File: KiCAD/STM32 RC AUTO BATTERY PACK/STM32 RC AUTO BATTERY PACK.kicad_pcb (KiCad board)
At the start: 2 copper layers, 147 x 100.2 mm, 9 parts, among them J1 Conn_01x02_Socket, J2 Conn_01x02_Socket, J3 Conn_01x02_Socket

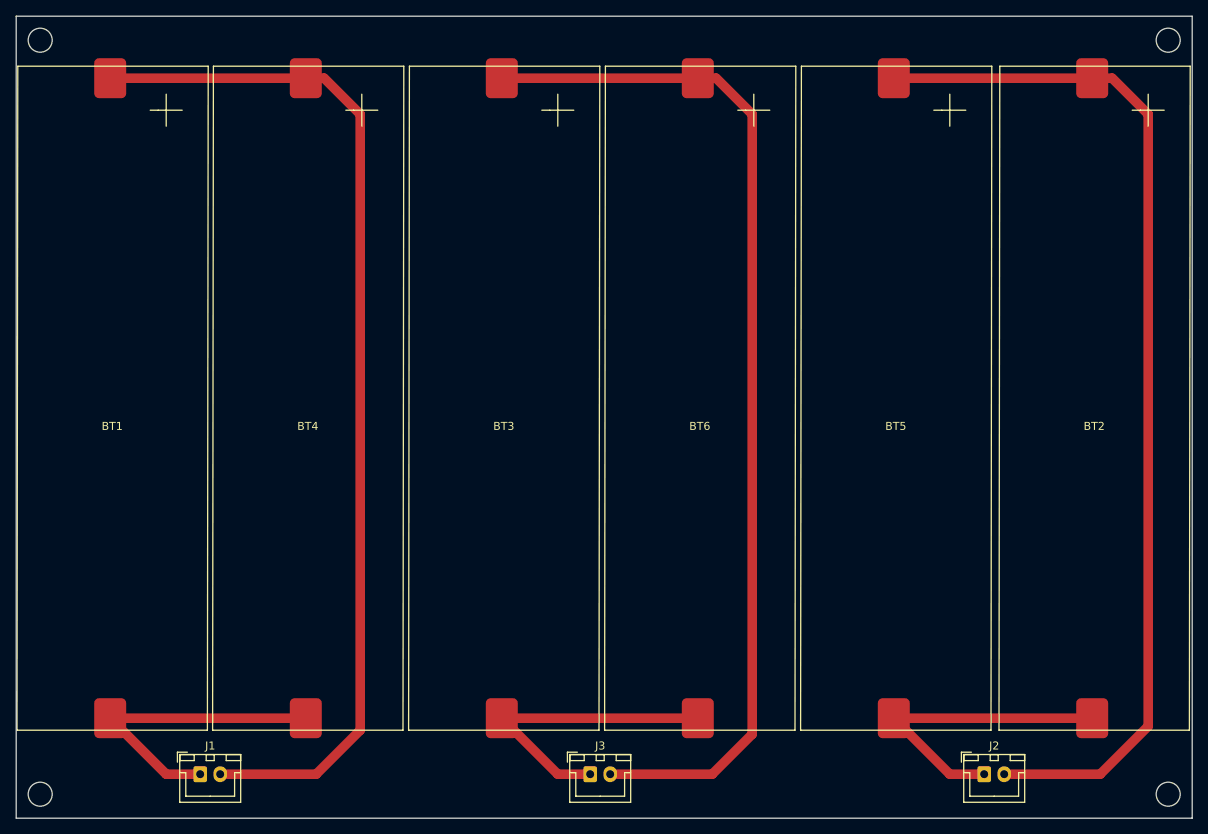
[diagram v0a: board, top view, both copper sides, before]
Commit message: ,
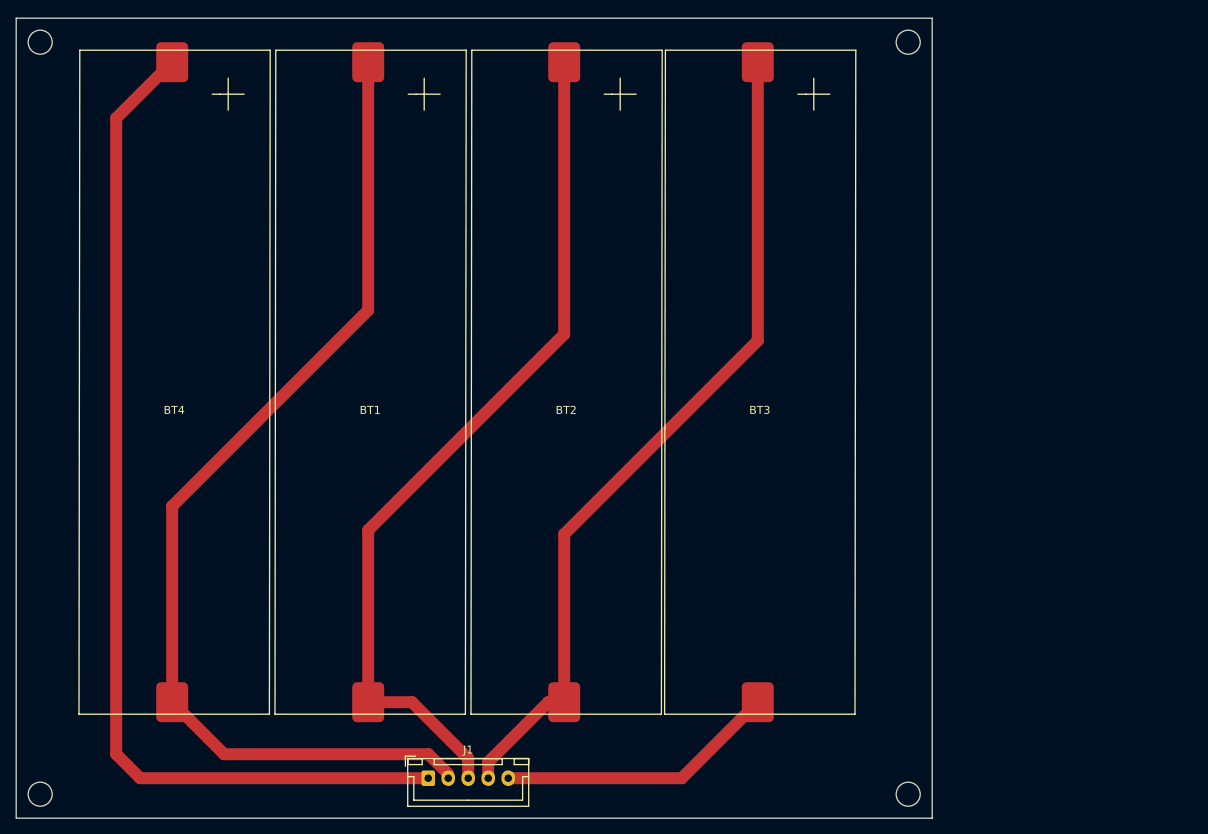
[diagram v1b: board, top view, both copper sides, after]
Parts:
- removed BT5, BT6: Battery_Cell, Batteryholder:21700 laskakit battery holder
- removed J2, J3: Conn_01x02_Socket, Connector_JST:JST_XH_B2B-XH-A_1x02_P2.50mm_Vertical
- J1: value Conn_01x02_Socket -> Conn_01x05_Socket; footprint Connector_JST:JST_XH_B2B-XH-A_1x02_P2.50mm_Vertical -> Connector_JST:JST_XH_B5B-XH-A_1x05_P2.50mm_Vertical
- moved BT2 66.0 mm to (137.0, 77.5)
- moved BT1 32.3 mm to (112.5, 77.5)
- moved BT3 32.1 mm to (161.2, 77.5)
- moved J1 28.5 mm to (120.0, 122.0)
- moved BT4 16.8 mm to (88.0, 77.5)
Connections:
- BT2 pad 1: Net-(BT2-+) -> Net-(BT1--)
- BT3 pad 1: Net-(BT3-+) -> Net-(BT2--)
- BT4 pad 1: Net-(BT1-+) -> Net-(BT4-+)
- BT4 pad 2: Net-(BT1--) -> Net-(BT1-+)
- J1 pad 1: Net-(BT1--) -> Net-(BT4-+)
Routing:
- net Net-(BT2-+): track 130.6 -> 0.00 mm
- net Net-(BT3-+): track 130.5 -> 0.00 mm
- net Net-(BT4-+): track 0.00 -> 129.6 mm
- net Net-(BT1--): track 38.6 -> 108.0 mm
- net Net-(BT2--): track 39.0 -> 104.6 mm
- net Net-(BT3--): track 38.4 -> 35.1 mm
- net Net-(BT1-+): track 129.9 -> 128.9 mm
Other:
- board size 147 x 100.2 mm -> 114.5 x 100 mm
